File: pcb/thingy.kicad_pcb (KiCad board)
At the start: 2 copper layers, 28 parts, among them J1 USB_B_Micro, J2 FLASH, J3 PROG, J4 I2C, SW1 POWER, SW2 RESET, U1 DW01A, U2 TP4056-B, U3 2x18650_holder, U4 FS8205A, U5 ESP-07

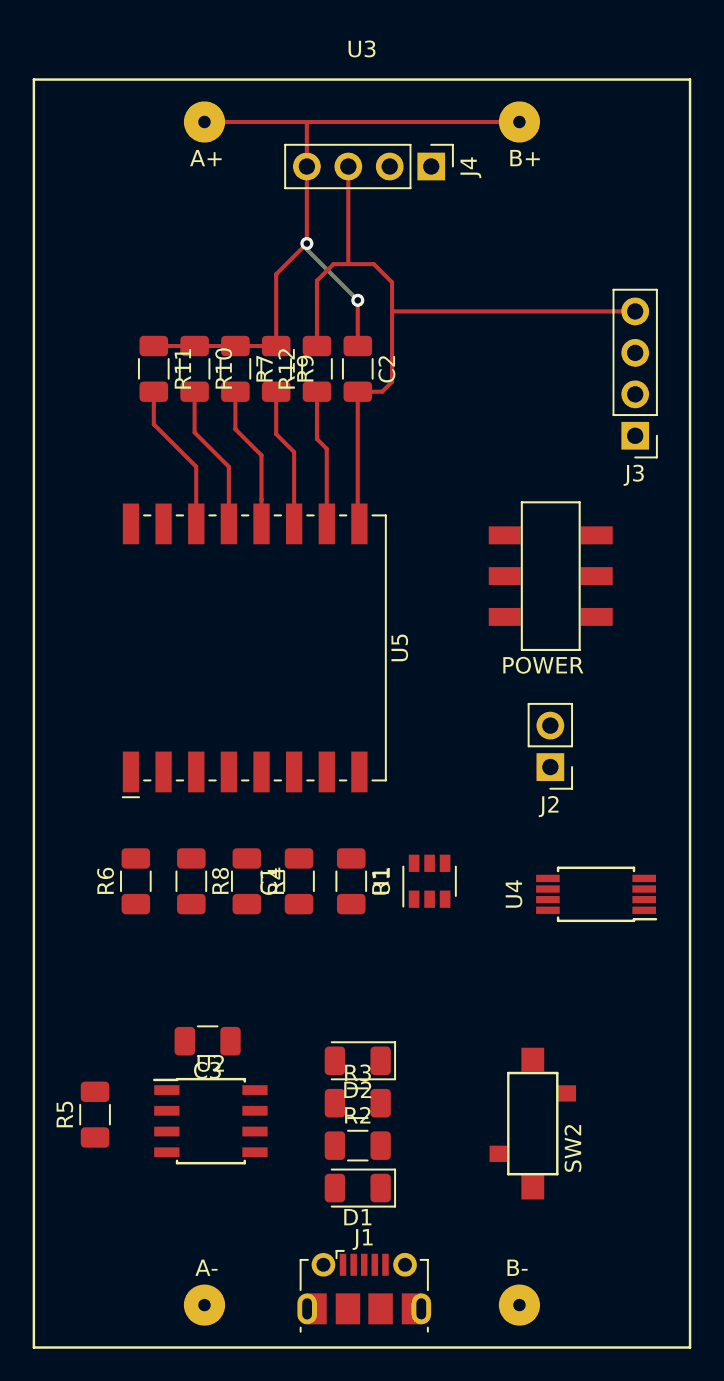
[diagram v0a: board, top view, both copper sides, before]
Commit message: almost finished work on pcb
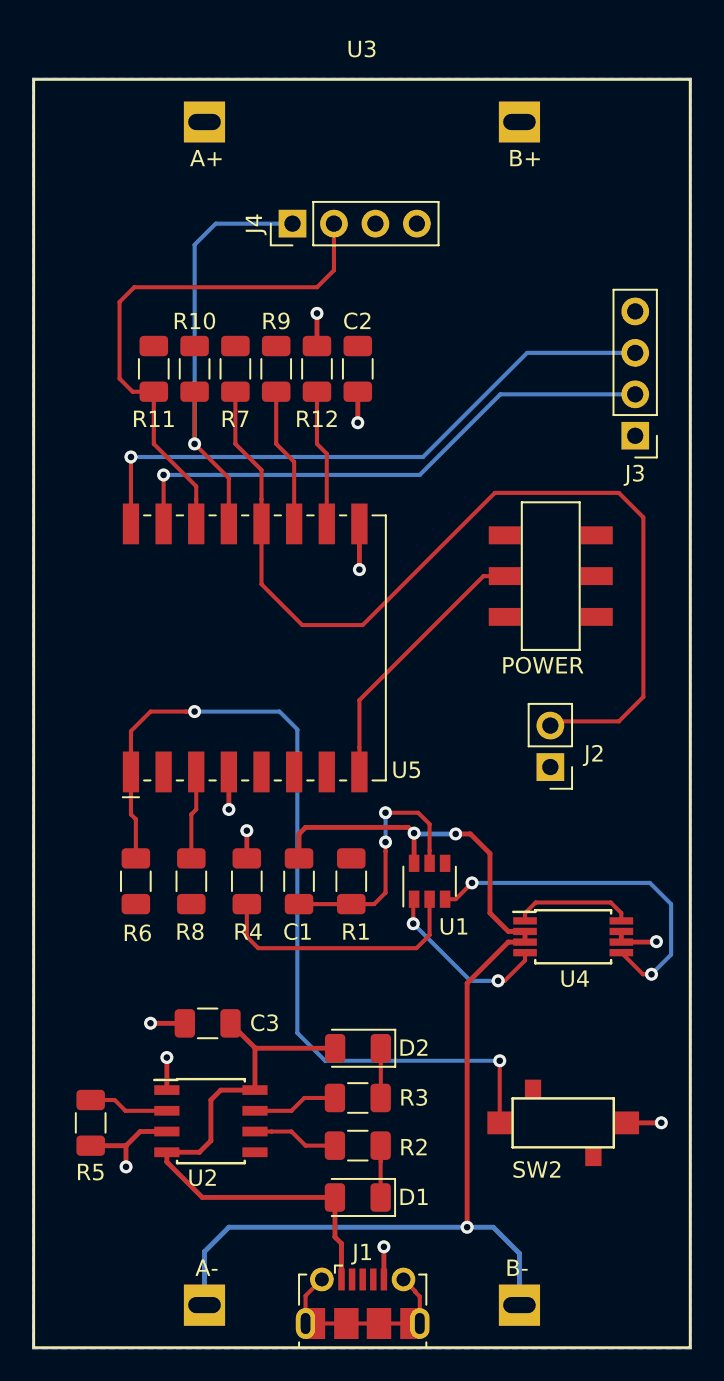
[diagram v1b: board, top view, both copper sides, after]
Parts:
- moved J4 9.19 mm to (116.0, 78.5), turned to 90 degrees
- moved U4 2.95 mm to (133.2, 122.2), turned to 0 degrees
- moved SW2 1.86 mm to (132.6, 133.6), turned to 180 degrees
- moved C3 1.09 mm to (110.8, 127.5)
- moved J1 0.90 mm to (120.3, 144.7)
- moved D2 0.77 mm to (120.0, 129.0)
- moved D1 0.58 mm to (120.0, 138.2)
- moved R5 0.57 mm to (103.6, 133.6), turned to 270 degrees
- moved R3 0.32 mm to (120.0, 132.1)
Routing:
- net BAT-: track 0.00 -> 69.4 mm, vias 0 -> 3
- net Net-(R6-Pad2): track 0.00 -> 54.6 mm, vias 0 -> 2
- net Net-(J2-Pad2): track 8.76 -> 58.3 mm
- net VCC: track 48.9 -> 0.00 mm, vias 2 -> 0
- net TXD: track 0.00 -> 37.6 mm, vias 0 -> 1
- net +5V: track 0.00 -> 35.1 mm
- net RXD: track 0.00 -> 33.9 mm, vias 0 -> 1
- net I2C_SCL: track 9.18 -> 33.1 mm
- net Net-(U1-Pad3): track 0.00 -> 22.0 mm, vias 0 -> 2
- net GND: track 47.0 -> 28.0 mm, vias 0 -> 11
- net I2C_SDA: track 8.97 -> 27.7 mm, vias 0 -> 1
- net Net-(SW1-Pad2): track 0.00 -> 16.4 mm
- net Net-(R4-Pad2): track 0.00 -> 16.0 mm
- net Net-(C1-Pad1): track 0.00 -> 15.9 mm, vias 0 -> 2
- net Net-(J1-Pad6): track 0.00 -> 12.0 mm
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- added copper zone on B.Cu, net GND
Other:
- board outline added: 40.4 x 77.8 mm
- net class POWER added: clearance 0.2, trace_width 0.3, via_dia 0.8, via_drill 0.4

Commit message: slightly more modifications
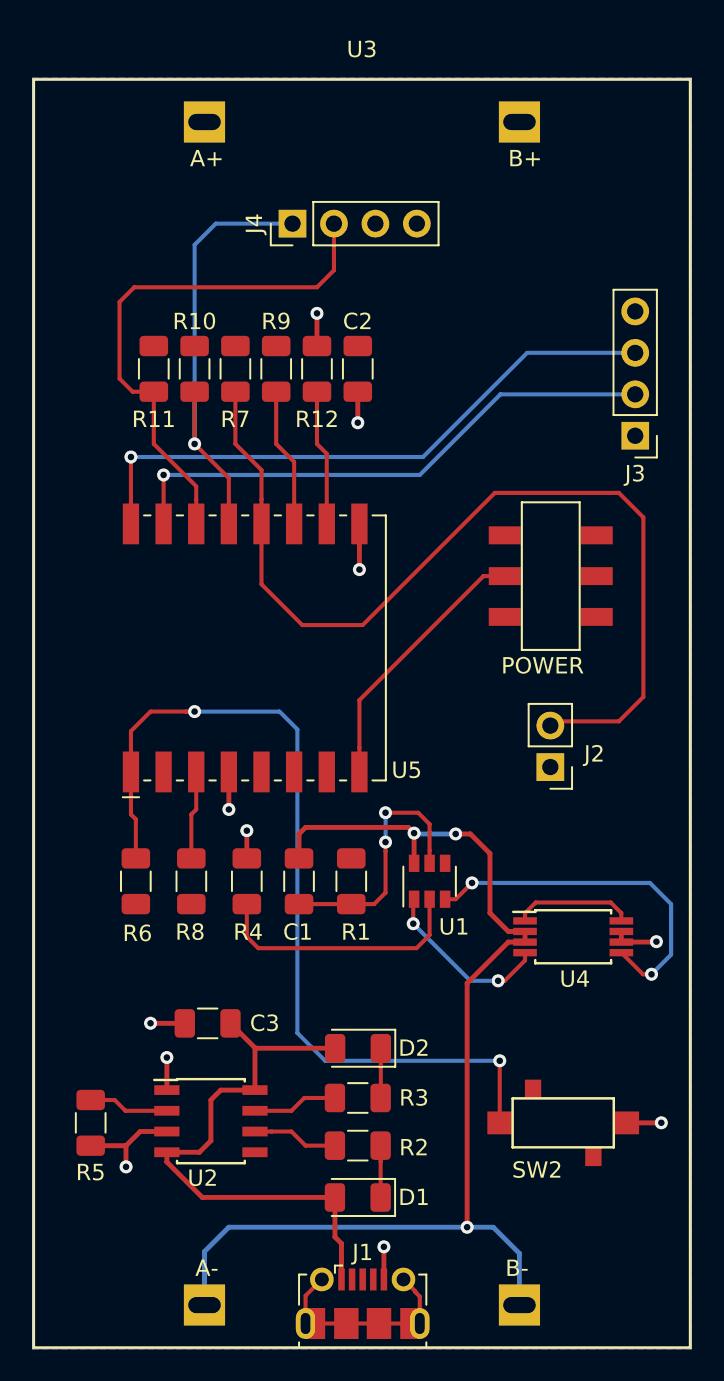
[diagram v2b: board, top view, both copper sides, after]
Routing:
- added copper zone on F.Cu, net VCC
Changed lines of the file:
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@@
+    )
+  )
+  (zone (net 9) (net_name VCC) (layer F.Cu) (hatch edge 0.508)
+    (connect_pads (clearance 0.508))
+    (min_thickness 0.254)
+    (fill yes (arc_segments 16) (thermal_gap 0.508) (thermal_bridge_width 0.508))
+    (polygon
+      (pts
+        (xy 100.08 69.6) (xy 100.08 147.44) (xy 140.43 147.44) (xy 140.43 69.6)
+      )
     )
   )
